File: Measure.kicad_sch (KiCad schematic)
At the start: 10 parts, among them U1 LMV7239M5, U7 AD8210

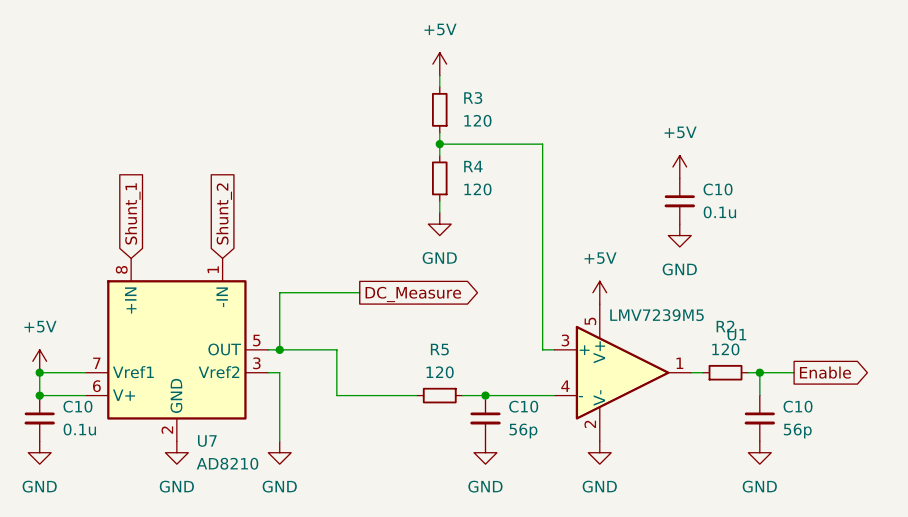
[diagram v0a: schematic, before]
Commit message: Стартовая версия
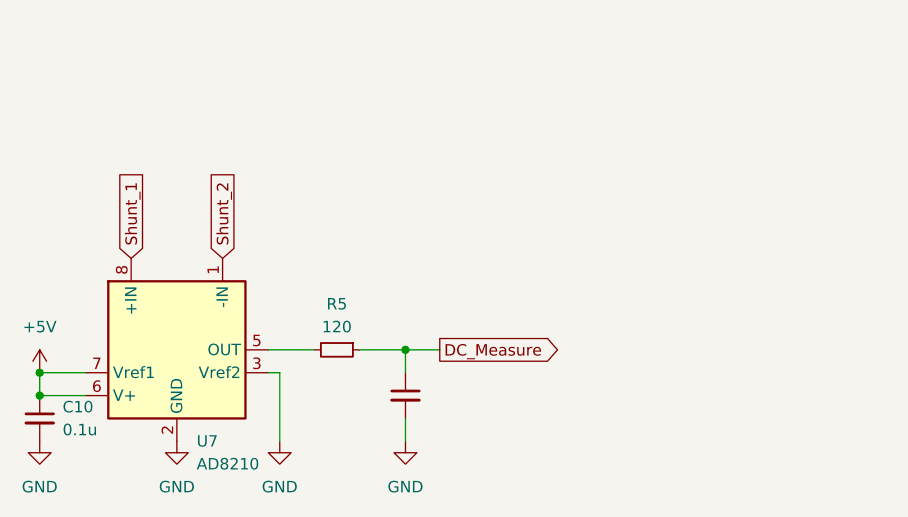
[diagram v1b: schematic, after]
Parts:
- removed C10: 0.1u, Capacitor_SMD:C_0805_2012Metric_Pad1.18x1.45mm_HandSolder, symbol Device:C_Small
- removed C10: 56p, Capacitor_SMD:C_0805_2012Metric_Pad1.18x1.45mm_HandSolder, symbol Device:C_Small
- removed R2, R3, R4: 120, Resistor_SMD:R_0805_2012Metric_Pad1.20x1.40mm_HandSolder, symbol Device:R_Small
- removed U1: LMV7239M5, Package_TO_SOT_SMD:SOT-353_SC-70-5, symbol Comparator:LMV7219M7
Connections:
- net DC_Measure: now also C10.1, R5.1; no longer R5.2, U7.5 (OUT)
- new net: R5.2, U7.5 (OUT)
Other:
- moved on the sheet: R5
